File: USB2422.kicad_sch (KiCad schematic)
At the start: 21 parts, among them U3 USB2422, Y1 Crystal_GND23_Small

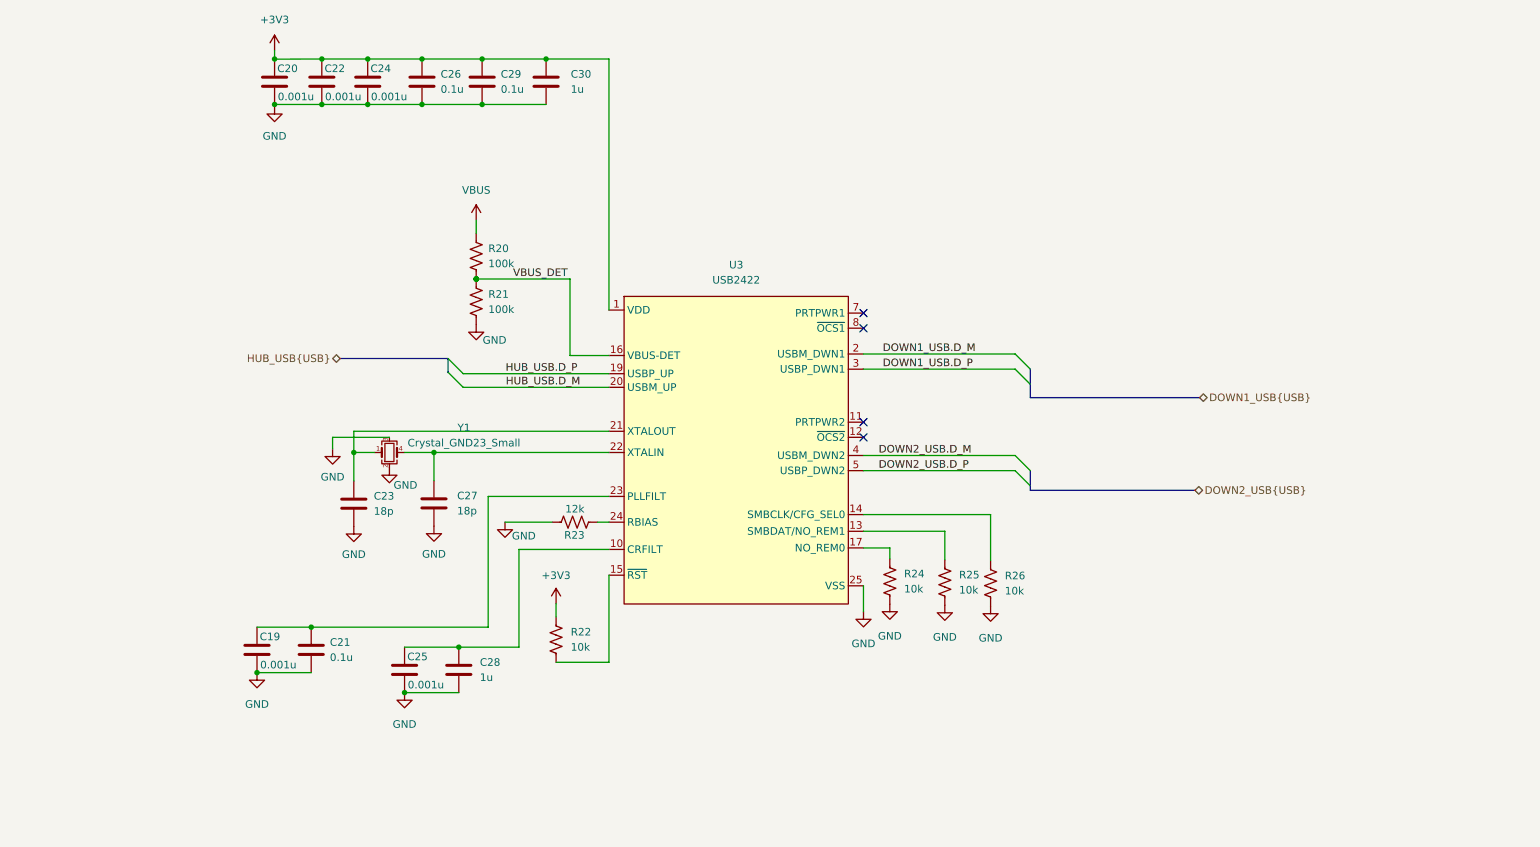
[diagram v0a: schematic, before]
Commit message: Pushing what i have now
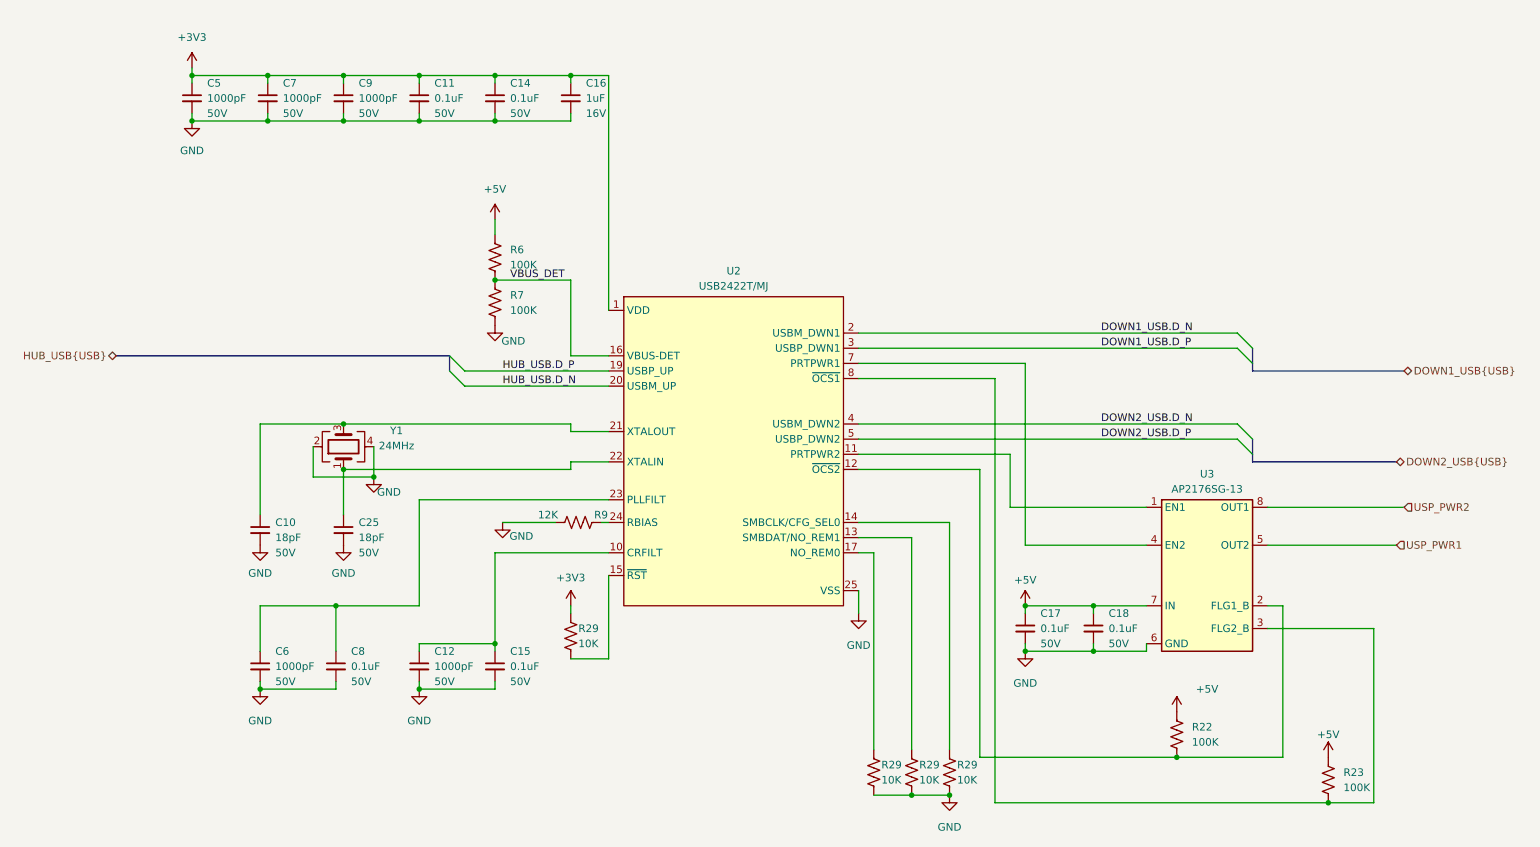
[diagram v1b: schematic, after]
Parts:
- removed C19, C20, C22, C24, C25: 0.001u, symbol Device:C
- removed C21, C26, C29: 0.1u, symbol Device:C
- removed C23, C27: 18p, symbol Device:C
- removed C28, C30: 1u, symbol Device:C
- removed R20, R21: 100k, symbol Device:R_US
- removed R22, R24, R25, R26: 10k, symbol Device:R_US
- removed R23: 12k, symbol Device:R_US
- removed U3: USB2422, symbol Misic:USB2422
- removed Y1: Crystal_GND23_Small, symbol Device:Crystal_GND23_Small
- added C10, C25: ${Capacitance}, Capacitor_SMD:C_0603_1608Metric_Pad1.08x0.95mm_HandSolder, symbol Rockerrobotics:Capacitors/1292-1494-1-ND
- added C11, C14, C15, C17, C18, C8: ${Capacitance}, Capacitor_SMD:C_0603_1608Metric_Pad1.08x0.95mm_HandSolder, symbol Rockerrobotics:Capacitors/1276-1935-1-ND
- added C12, C5, C6, C7, C9: ${Capacitance}, Capacitor_SMD:C_0603_1608Metric_Pad1.08x0.95mm_HandSolder, symbol Rockerrobotics:Capacitors/1276-1018-1-ND
- added C16: ${Capacitance}, Capacitor_SMD:C_0603_1608Metric_Pad1.08x0.95mm_HandSolder, symbol Rockerrobotics:Capacitors/1276-1034-1-ND
- added R22, R23, R6, R7: ${Resistance}, Resistor_SMD:R_0805_2012Metric_Pad1.20x1.40mm_HandSolder, symbol Rockerrobotics:Resistors/RMCF0805FT100KCT-ND
- added R29 (x4): ${Resistance}, Resistor_SMD:R_0805_2012Metric_Pad1.20x1.40mm_HandSolder, symbol Rockerrobotics:Resistors/RNCP0805FTD10K0CT-ND
- added R9: ${Resistance}, Resistor_SMD:R_0805_2012Metric_Pad1.20x1.40mm_HandSolder, symbol Rockerrobotics:Resistors/311-12KARCT-ND
- added U2: ${MPN}, Rockerrobotics:SQFN24_4X4MC_MCH, symbol Rockerrobotics:Integrated Circuits/USB2422T/MJCT-ND
- added U3: ${MPN}, Rockerrobotics:Diodes-SO8, symbol Rockerrobotics:Integrated Circuits/AP2176SGDICT-ND
- added Y1: 24MHz, Crystal:Crystal_SMD_2520-4Pin_2.5x2.0mm, symbol Rockerrobotics:Oscillator/XC2641CT-ND
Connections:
- net +3V3: now also C11.1, C14.1, C16.1, C5.1, C7.1, C9.1, R29.1, U2.1 (VDD), U2.18 (VDD), U2.9 (VDD)
- net DOWN1_USB.D_P: now also U2.3 (USBP_DWN1)
- net DOWN2_USB.D_P: now also U2.5 (USBP_DWN2)
- net GND: now also C10.2, C11.2, C12.2, C14.2, C15.2, C16.2, C17.2, C18.2, C25.2, C5.2, C6.2, C7.2, C8.2, C9.2, R29.2, R29.2, R29.2, R7.2, R9.1, U2.25 (VSS), U3.6 (GND), Y1.2, Y1.4
- net HUB_USB.D_P: now also U2.19 (USBP_UP)
- net VBUS_DET: now also R6.2, R7.1, U2.16 (VBUS-DET)
- new net: R9.2, U2.24 (RBIAS)
- new net: R29.2, U2.15 (~{RST})
- new net: R22.2, U2.12 (~{OCS2}), U3.2 (FLG1_B)
- new net: R23.2, U2.8 (~{OCS1}), U3.3 (FLG2_B)
- new net: C10.1, U2.21 (XTALOUT), Y1.3
- new net: R29.1, U2.17 (NO_REM0)
- new net: R29.1, U2.13 (SMBDAT/NO_REM1)
- new net: C25.1, U2.22 (XTALIN), Y1.1
- new net: C6.1, C8.1, U2.23 (PLLFILT)
- new net: R29.1, U2.14 (SMBCLK/CFG_SEL0)
- new net: C12.1, C15.1, U2.10 (CRFILT)
- new net: U2.11 (PRTPWR2), U3.1 (EN1)
- new net: U2.7 (PRTPWR1), U3.4 (EN2)
- new net +5V: C17.1, C18.1, R22.1, R23.1, R6.1, U3.7 (IN)
- new net DOWN1_USB.D_N: U2.2 (USBM_DWN1)
- new net DOWN2_USB.D_N: U2.4 (USBM_DWN2)
- new net HUB_USB.D_N: U2.20 (USBM_UP)
- new net USP_PWR1: U3.5 (OUT2)
- new net USP_PWR2: U3.8 (OUT1)
- no-connect marks 4 -> 0
